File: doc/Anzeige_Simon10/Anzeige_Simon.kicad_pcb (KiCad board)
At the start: 2 copper layers, 50 x 37 mm, 25 parts, among them J1 I2C, J2 Daten, J3 MoGND, J4 Vcc, J5 AnzByte, U1 74HC688, U2 PCF8574P, U3 SFH617

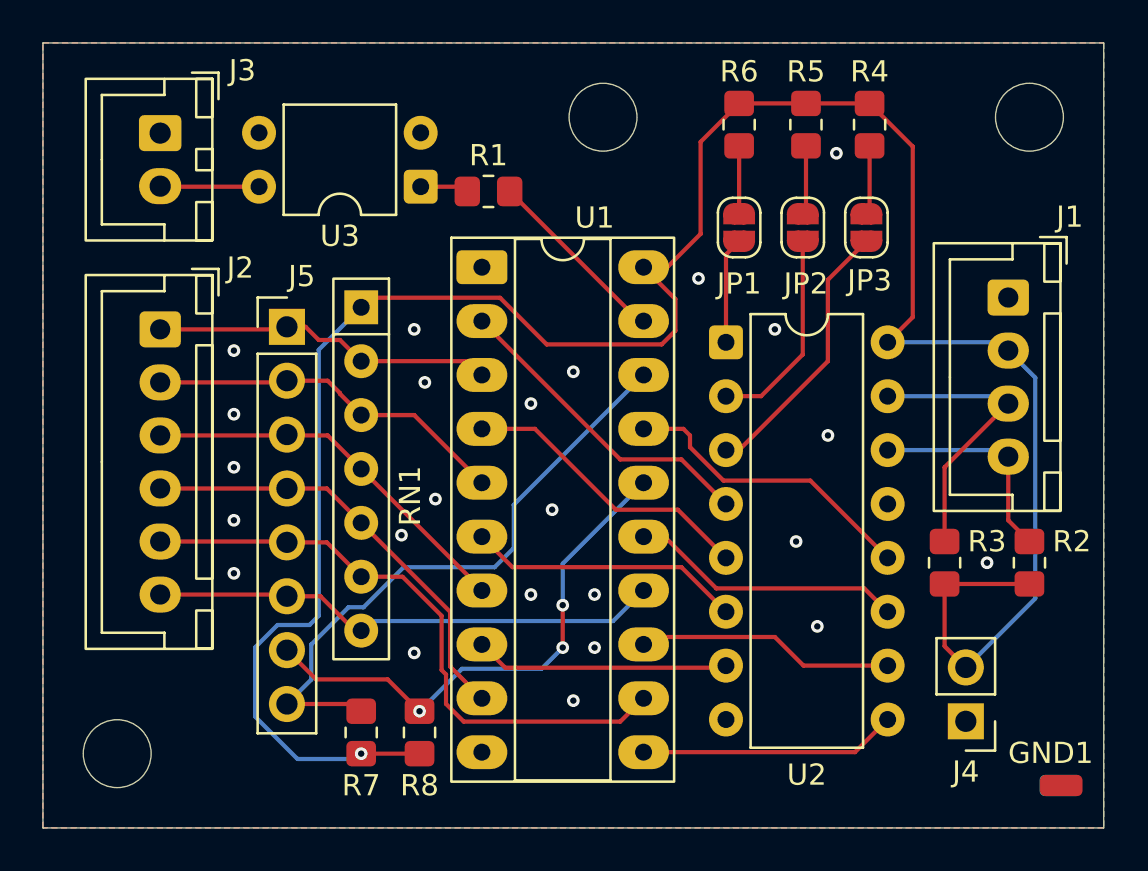
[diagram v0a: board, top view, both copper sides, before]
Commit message: Update files
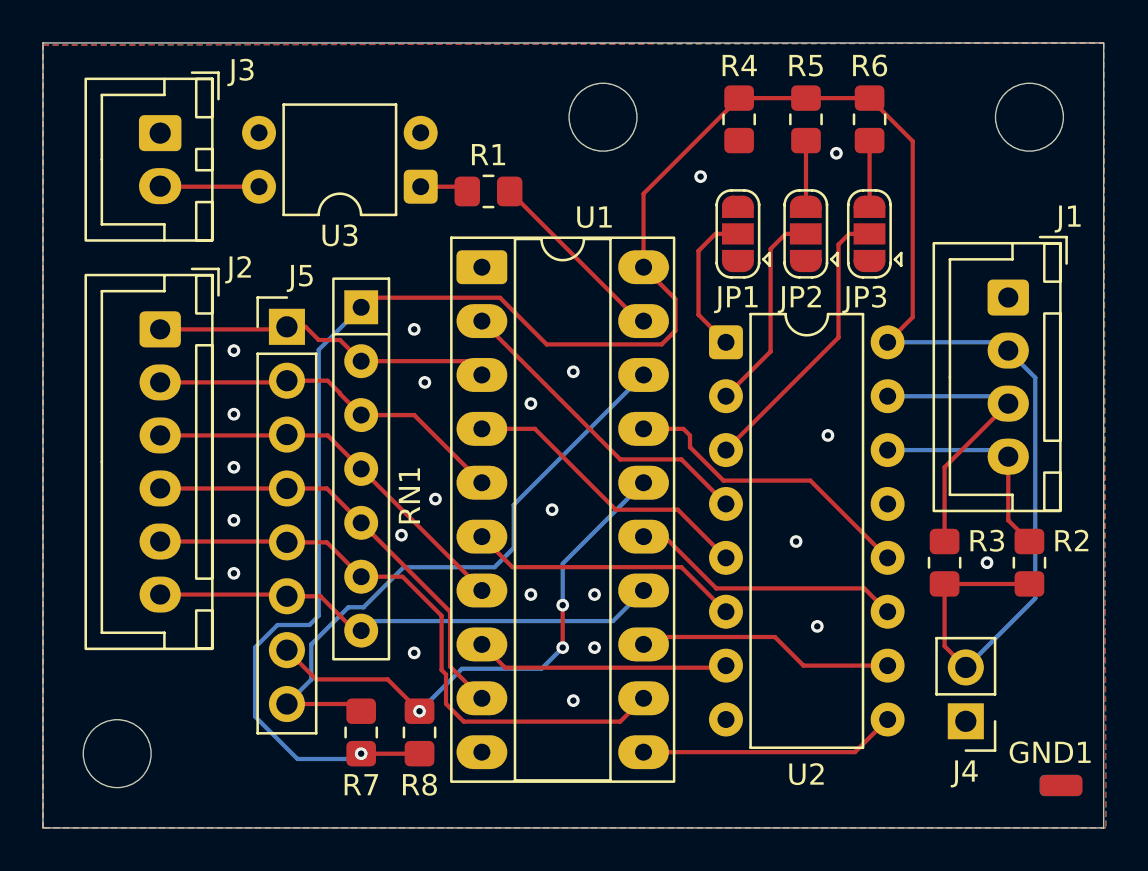
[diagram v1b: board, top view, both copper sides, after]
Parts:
- JP1, JP2, JP3: value ~ -> Jumper_3_Open; footprint Jumper:SolderJumper-2_P1.3mm_Open_RoundedPad1.0x1.5mm -> Jumper:SolderJumper-3_P1.3mm_Open_RoundedPad1.0x1.5mm
- R1: value 330 -> 220
- moved JP2 0.33 mm to (70.5, 56.5), turned to 90 degrees
- moved JP3 0.33 mm to (73.5, 56.5), turned to 90 degrees
- moved JP1 0.31 mm to (67.3, 56.5), turned to 90 degrees
- moved R4 0.25 mm to (67.3, 51.1)
- moved R5 0.25 mm to (70.5, 51.1)
- moved R6 0.25 mm to (73.5, 51.1)
- renumbered R6 to R4, R4 to R6
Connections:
- net +5V renamed Vcc
- JP1 pad 1: Net-(JP1-A) -> GND
- JP1 pad 2: Net-(JP1-B) -> A0
- JP2 pad 1: Net-(JP2-A) -> GND
- JP2 pad 2: Net-(JP2-B) -> A1
- JP3 pad 1: Net-(JP3-A) -> GND
- JP3 pad 2: Net-(JP3-B) -> A2
- R4 pad 2: Net-(JP1-A) -> Net-(JP1-B)
- R5 pad 2: Net-(JP2-A) -> Net-(JP2-B)
- R6 pad 2: Net-(JP3-A) -> Net-(JP3-B)
- U2 pad 1: Net-(JP1-B) -> A0
- U2 pad 2: Net-(JP2-B) -> A1
- U2 pad 3: Net-(JP3-B) -> A2
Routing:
- net A2: track 0.00 -> 13.6 mm
- net Net-(JP3-B): track 12.9 -> 3.10 mm
- net A1: track 0.00 -> 9.76 mm
- net A0: track 0.00 -> 7.04 mm
- net Net-(JP2-B): track 9.77 -> 3.10 mm
- net Net-(JP1-B): track 5.02 -> 0.00 mm
- net Net-(JP3-A): track 3.26 -> 0.00 mm
- net Net-(JP2-A): track 3.26 -> 0.00 mm
- net Net-(JP1-A): track 3.20 -> 0.00 mm
- net Vcc: track 111.8 -> 112.8 mm
- net GND: vias 24 -> 23

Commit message: Add files via upload
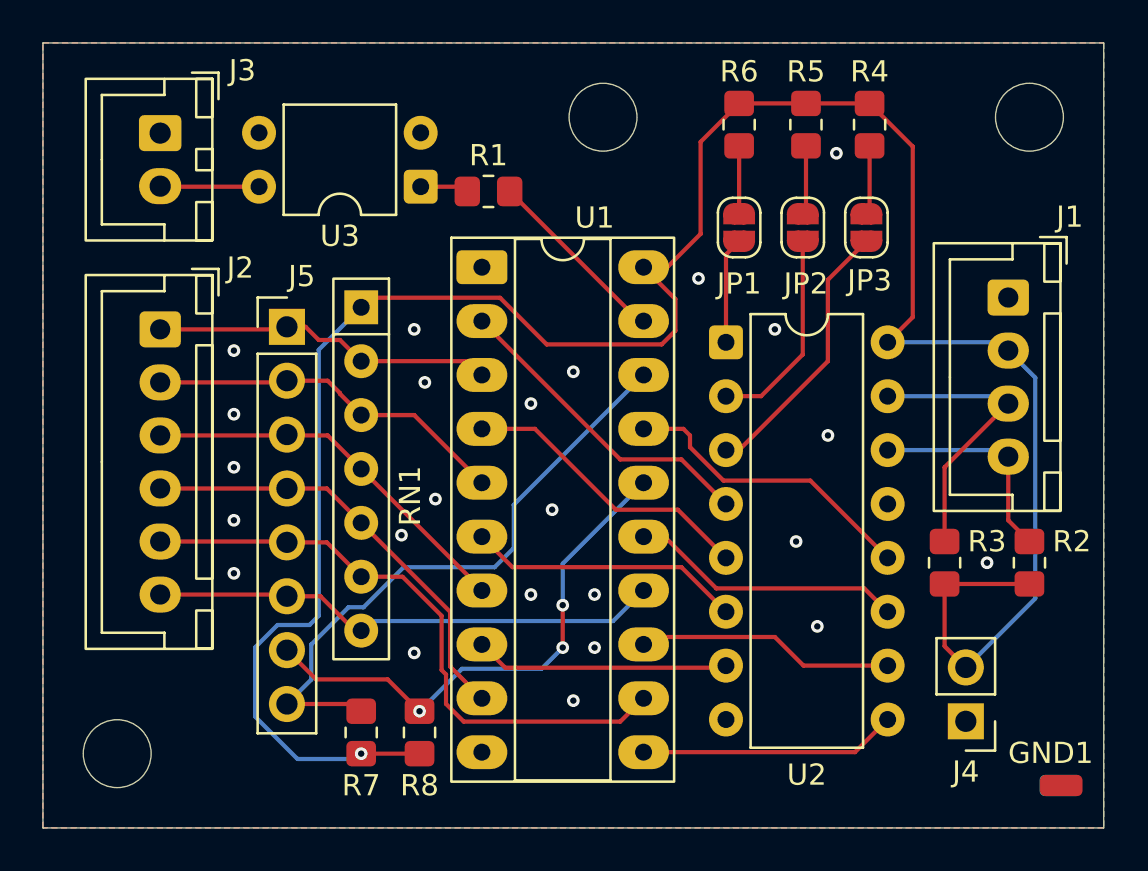
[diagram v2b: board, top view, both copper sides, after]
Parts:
- JP1, JP2, JP3: value Jumper_3_Open -> ~; footprint Jumper:SolderJumper-3_P1.3mm_Open_RoundedPad1.0x1.5mm -> Jumper:SolderJumper-2_P1.3mm_Open_RoundedPad1.0x1.5mm
- R1: value 220 -> 330
- moved JP2 0.33 mm to (70.3, 56.2), turned to -90 degrees
- moved JP3 0.33 mm to (73.3, 56.2), turned to -90 degrees
- moved JP1 0.31 mm to (67.3, 56.2), turned to -90 degrees
- moved R4 0.25 mm to (73.5, 51.4)
- moved R5 0.25 mm to (70.5, 51.4)
- moved R6 0.25 mm to (67.3, 51.4)
- renumbered R6 to R4, R4 to R6
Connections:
- net A0 renamed Net-(JP1-B)
- net A1 renamed Net-(JP2-B)
- net A2 renamed Net-(JP3-B)
- net Vcc renamed +5V
- JP1 pad 1: GND -> Net-(JP1-A)
- JP2 pad 1: GND -> Net-(JP2-A)
- JP3 pad 1: GND -> Net-(JP3-A)
- R4 pad 2: Net-(JP3-B) (its old number) -> Net-(JP3-A)
- R5 pad 2: Net-(JP2-B) (its old number) -> Net-(JP2-A)
- R6 pad 2: Net-(JP1-B) (its old number) -> Net-(JP1-A)
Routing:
- net Net-(JP3-A): track 0.00 -> 3.26 mm
- net Net-(JP2-A): track 0.00 -> 3.26 mm
- net Net-(JP1-A): track 0.00 -> 3.20 mm
- net Net-(JP3-B) (its old number): track 3.10 -> 0.00 mm
- net Net-(JP2-B) (its old number): track 3.10 -> 0.00 mm
- net Net-(JP1-B): track 7.04 -> 5.02 mm
- net +5V: track 112.8 -> 111.8 mm
- net Net-(JP3-B): track 13.6 -> 12.9 mm
- net GND: vias 23 -> 24
